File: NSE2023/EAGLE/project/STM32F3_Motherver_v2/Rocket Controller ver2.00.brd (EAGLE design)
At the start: 35.5 x 35.2 mm, 23 parts

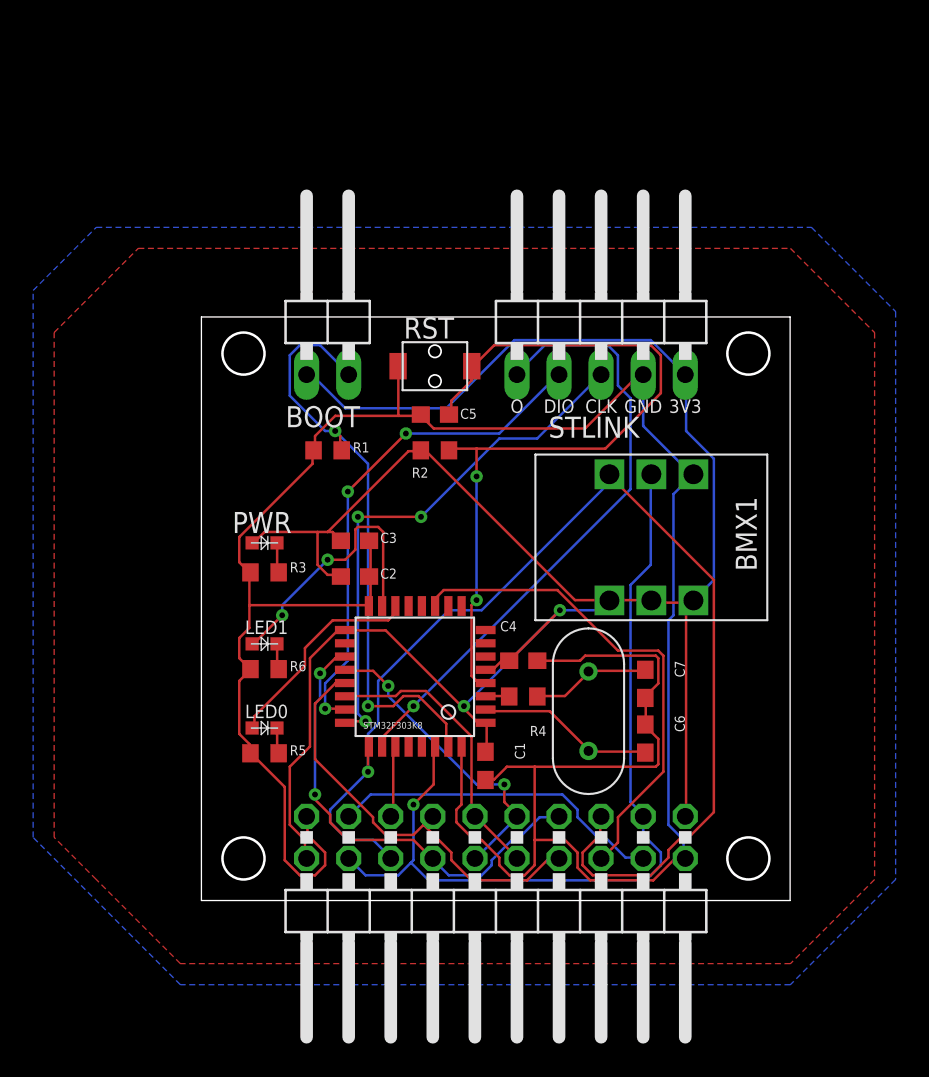
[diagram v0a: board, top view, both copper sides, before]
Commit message: create final board NSE2023
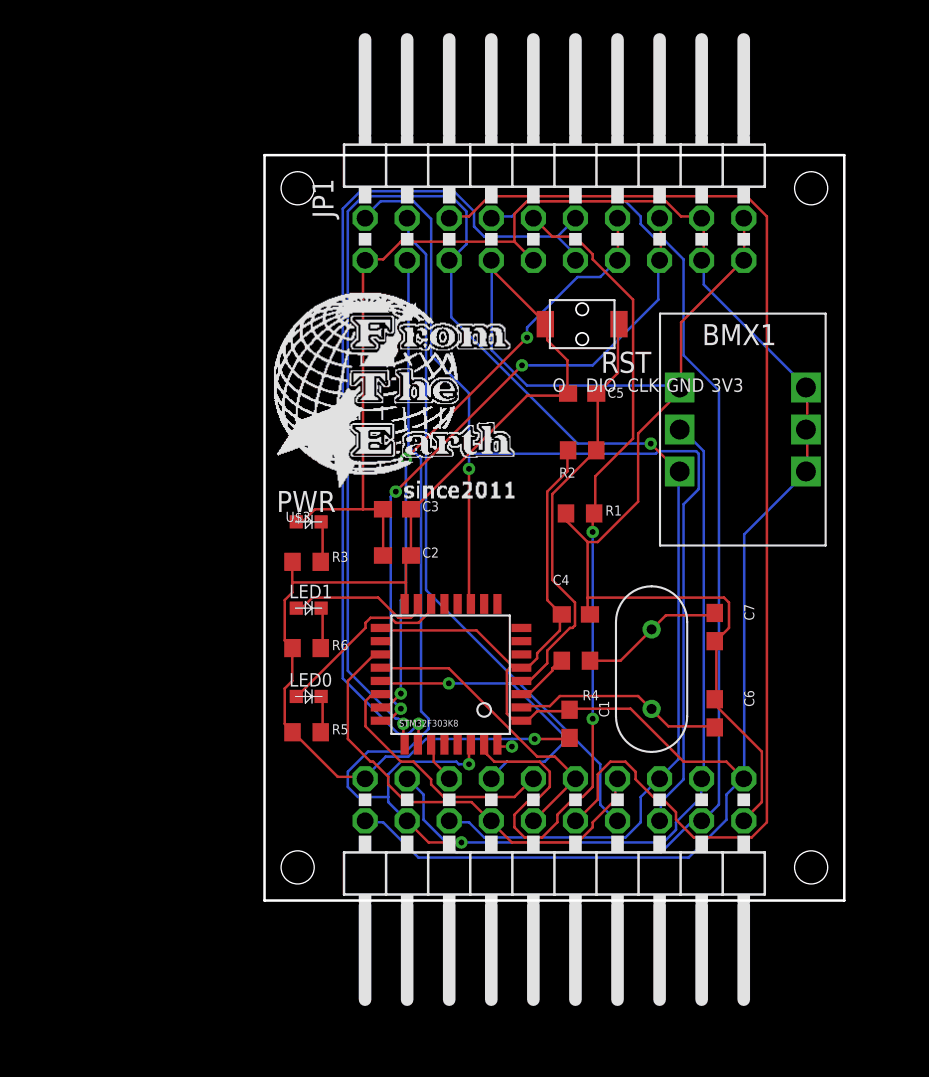
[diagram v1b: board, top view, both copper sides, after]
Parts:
- removed BOOT: (no value), pinhead:1X02/90
- removed STLINK: (no value), pinhead:1X05/90
- added JP1: (no value), pinhead:2X10/90
- added U$3: F.T.E.LOGO, logo:LOGO
- moved R1 15.7 mm to (19.1, 23.4)
- moved BMX1 10.7 mm to (23.9, 35.4), turned to 0 degrees
- moved RST 9.25 mm to (19.2, 34.8)
- moved C5 8.98 mm to (19.2, 30.6)
- moved R2 8.89 mm to (19.2, 27.2)
- moved C1 5.68 mm to (18.4, 10.7)
- moved C7 5.42 mm to (27.2, 16.5)
- moved CRY1 4.58 mm to (23.4, 14.0)
- moved C6 4.46 mm to (27.2, 11.3)
- moved C4 4.23 mm to (18.8, 17.3)
- moved JP3 4.20 mm to (17.5, 1.00)
- moved R4 3.84 mm to (18.8, 14.5)
- moved LED1 3.43 mm to (2.67, 17.7)
- moved LED0 3.28 mm to (2.67, 12.3)
- moved C3 3.18 mm to (8.00, 23.6)
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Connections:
- removed net N$11: JP3.17, JP3.4
- new net +5V: JP1.8, JP3.17, JP3.4
- new net FPRAW: JP1.6, JP3.10
- new net SW: JP1.4, JP3.8
- net +3V3: now also JP1.1, JP1.17, JP1.18, JP1.9; no longer BOOT.1, STLINK.5
- net BIT1: no longer JP3.10
- net BIT2: no longer JP3.8
- net BOOT0: now also JP1.10; no longer BOOT.2
- net GND: now also JP1.19, JP1.20, JP1.7; no longer STLINK.4
- net PWM: now also JP1.2
- net SCL: now also JP1.5
- net SDA: now also JP1.3
- net SWCLK: now also JP1.15, JP1.16; no longer STLINK.3
- net SWDIO: now also JP1.13, JP1.14; no longer STLINK.2
- net SWO: now also JP1.11, JP1.12; no longer STLINK.1
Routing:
- net FPRAW: track 0.00 -> 73.5 mm
- net +5V: track 0.00 -> 70.4 mm
- net SW: track 0.00 -> 41.7 mm
- net SDA: track 52.9 -> 90.8 mm, vias 1 -> 2
- net PWM: track 29.9 -> 66.3 mm, vias 0 -> 1
- net SCL: track 71.7 -> 100.7 mm, vias 1 -> 2
- net NRST: track 47.1 -> 25.6 mm, vias 2 -> 0
- net N$11: track 20.2 -> 0.00 mm
- net +3V3: track 138.3 -> 158.4 mm, vias 2 -> 0
- net GND: track 158.0 -> 138.8 mm, vias 0 -> 2
- net BOOT0: track 36.6 -> 54.6 mm
- net SWO: track 37.3 -> 54.3 mm
- net SWCLK: track 32.1 -> 40.7 mm
- net BIT2: track 26.4 -> 18.2 mm, vias 0 -> 1
- net LED1: track 16.5 -> 8.71 mm, vias 2 -> 0
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- removed copper zone on layer 1, net GND
- removed copper zone on layer 16, net GND
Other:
- board size 35.5 x 35.2 mm -> 35 x 45 mm

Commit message: www
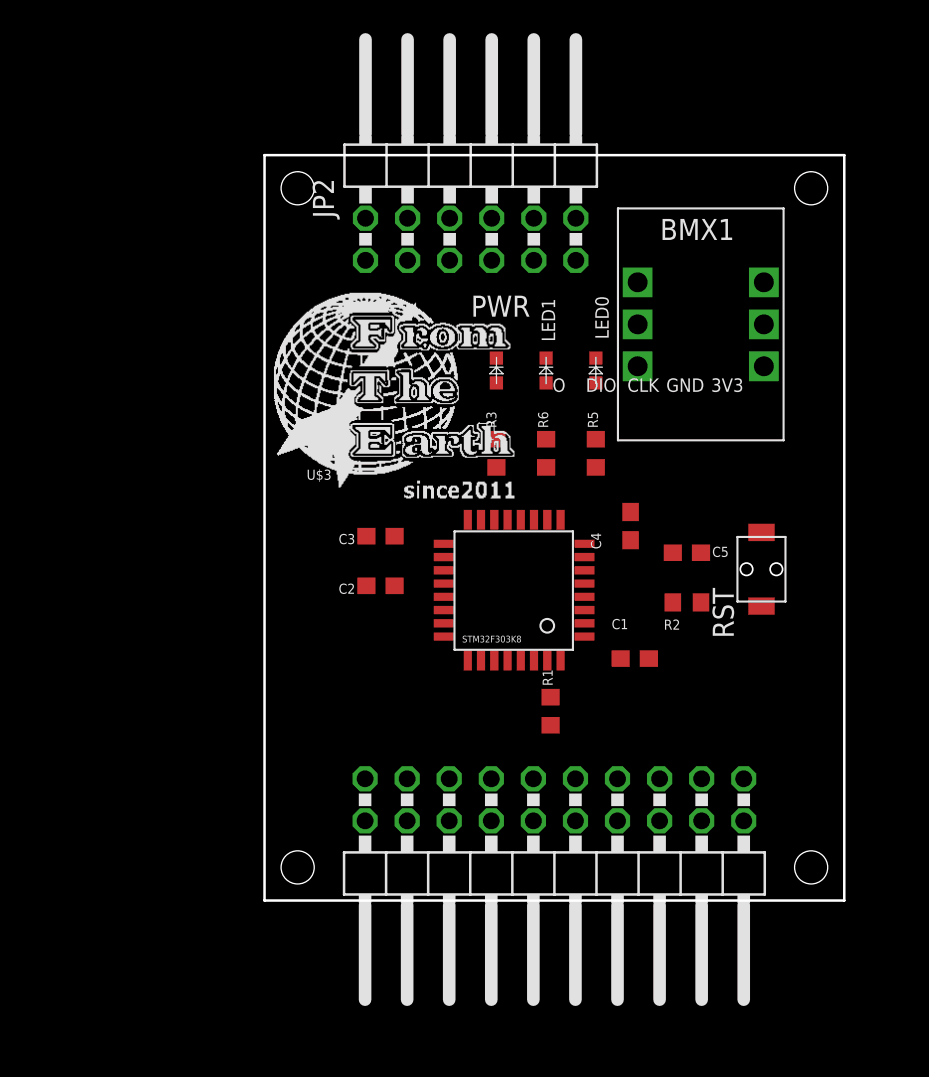
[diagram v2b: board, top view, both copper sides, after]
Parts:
- removed C6, C7: 30pF, rcl:C1608
- removed CRY1: (no value), Crystal:CRYSTAL
- removed JP1: (no value), pinhead:2X10/90
- removed R4: DNF, rcl:R0603
- added JP2: (no value), pinhead:2X06/90
- moved LED0 26.2 mm to (20.0, 32.0), turned to 90 degrees
- moved R5 24.3 mm to (20.0, 27.0), turned to 90 degrees
- moved LED1 20.3 mm to (17.0, 32.0), turned to 90 degrees
- moved R6 18.6 mm to (17.0, 27.0), turned to 90 degrees
- moved RST 18.3 mm to (30.0, 20.0), turned to 180 degrees
- moved PWR 14.6 mm to (14.0, 32.0), turned to 90 degrees
- moved R3 13.2 mm to (14.0, 27.0), turned to 90 degrees
- moved R1 12.1 mm to (17.3, 11.4), turned to 270 degrees
- moved C5 11.5 mm to (25.5, 21.0)
- moved R2 11.1 mm to (25.5, 18.0)
- moved BMX1 6.84 mm to (21.3, 41.8)
- moved U$1 6.35 mm to (18.7, 23.0)
- moved C4 6.27 mm to (22.1, 22.6), turned to 90 degrees
- moved C1 5.57 mm to (22.4, 14.6), turned to 0 degrees
- moved C2 2.08 mm to (7.00, 19.0), turned to 180 degrees
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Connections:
- removed net N$3: C7.1, CRY1.P$2, R4.1
- net +3V3: now also JP2.9; no longer JP1.1, JP1.17, JP1.18, JP1.9
- net +5V: now also JP2.2; no longer JP1.8
- net BOOT0: no longer JP1.10
- net FPRAW: now also JP2.12; no longer JP1.6
- net GND: now also JP2.11; no longer C6.2, C7.2, JP1.19, JP1.20, JP1.7
- net NRST: now also JP2.8
- net OSC_IN: no longer C6.1, CRY1.P$1
- net OSC_OUT: no longer R4.2
- net PWM: now also JP2.1; no longer JP1.2
- net SCL: now also JP2.6; no longer JP1.5
- net SDA: now also JP2.4; no longer JP1.3
- net SW: now also JP2.10; no longer JP1.4
- net SWCLK: now also JP2.7; no longer JP1.15, JP1.16
- net SWDIO: now also JP2.5; no longer JP1.13, JP1.14
- net SWO: now also JP2.3; no longer JP1.11, JP1.12
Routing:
- net +3V3: track 158.4 -> 0.00 mm
- net GND: track 138.8 -> 0.00 mm, vias 2 -> 0
- net SCL: track 100.7 -> 0.00 mm, vias 2 -> 0
- net SDA: track 90.8 -> 0.00 mm, vias 2 -> 0
- net FPRAW: track 73.5 -> 0.00 mm
- net +5V: track 70.4 -> 0.00 mm
- net PWM: track 66.3 -> 0.00 mm, vias 1 -> 0
- net BOOT0: track 54.6 -> 0.00 mm, vias 2 -> 0
- net SWO: track 54.3 -> 0.00 mm, vias 1 -> 0
- net SW: track 41.7 -> 0.00 mm
- net SWCLK: track 40.7 -> 0.00 mm, vias 3 -> 0
- net SWDIO: track 36.6 -> 0.00 mm, vias 3 -> 0
- net LOGRX: track 27.8 -> 0.00 mm
- net NRST: track 25.6 -> 0.00 mm
- net BIT2: track 18.2 -> 0.00 mm, vias 1 -> 0
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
